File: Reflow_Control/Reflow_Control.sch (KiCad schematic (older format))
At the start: 36 parts

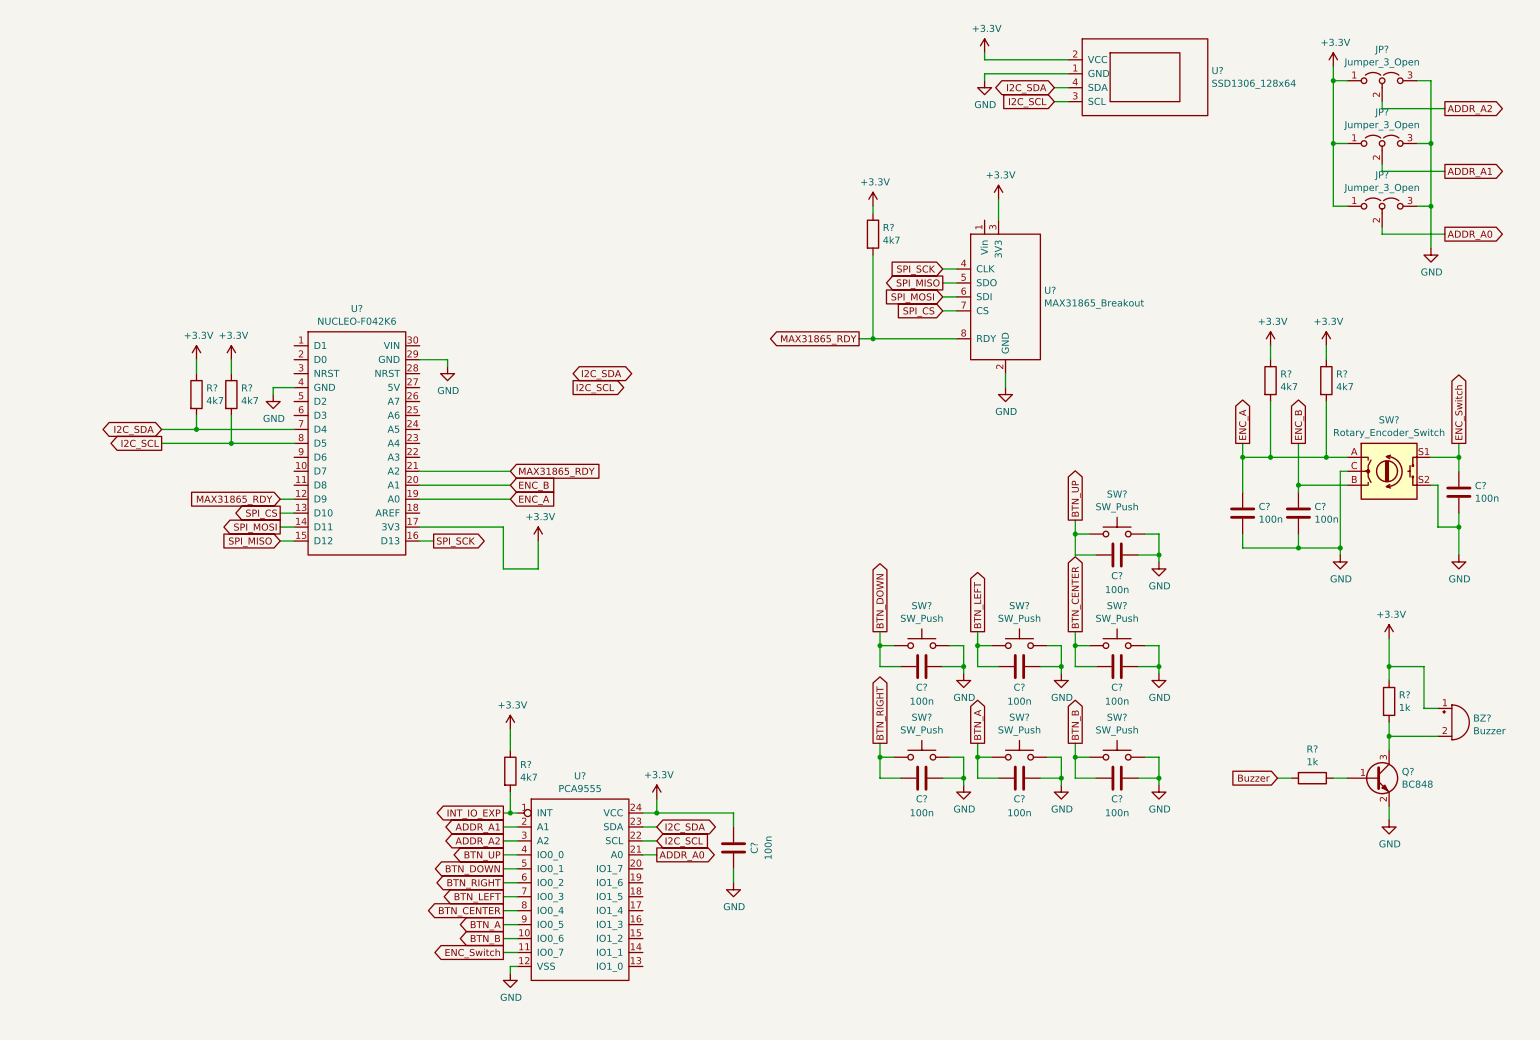
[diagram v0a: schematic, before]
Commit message: work on naming
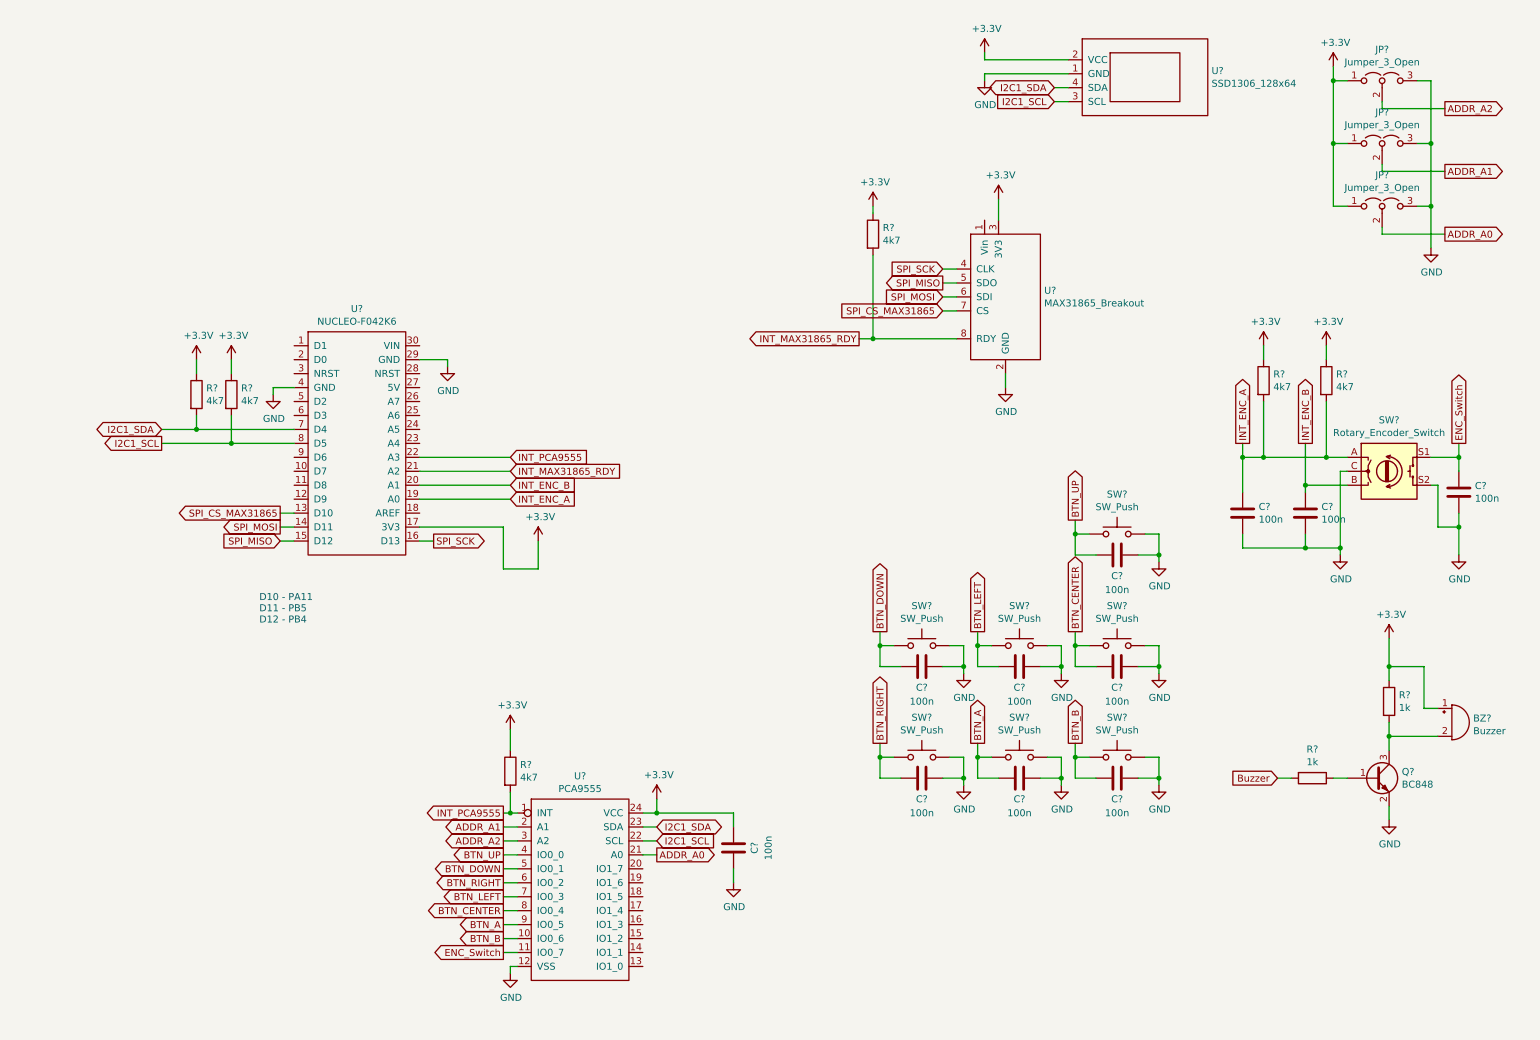
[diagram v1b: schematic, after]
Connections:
- net INT_IO_EXP is gone; now on net INT_PCA9555: R?.2, U?.1 (INT)
- net INT_PCA9555: now reaches U?.22 (A3)
- net ENC_A renamed INT_ENC_A
- net ENC_B renamed INT_ENC_B
- net I2C_SCL renamed I2C1_SCL
- net I2C_SDA renamed I2C1_SDA
- net MAX31865_RDY renamed INT_MAX31865_RDY
- net INT_MAX31865_RDY: no longer U?.12 (D9)
- net SPI_CS renamed SPI_CS_MAX31865
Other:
- note added: "D10 - PA11\nD11 - PB5\nD12 - PB4\n"
- moved on the sheet: C?, R?
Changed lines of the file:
@@
 L Device:R R?
 U 1 1 5F9458E6
-P 9450 3150
-F 0 "R?" H 9520 3196 50  0000 L CNN
-F 1 "4k7" H 9520 3105 50  0000 L CNN
-F 2 "Resistor_SMD:R_1206_3216Metric_Pad1.42x1.75mm_HandSolder" V 9380 3150 50  0001 C CNN
-F 3 "~" H 9450 3150 50  0001 C CNN
-F 4 "Rhom" H 9450 3150 50  0001 C CNN "Man"
-F 5 "KTR18EZPF4701" H 9450 3150 50  0001 C CNN "Man no"
-F 6 "Digikey" H 9450 3150 50  0001 C CNN "Dist"
-F 7 "RHM4.7KAICT-ND" H 9450 3150 50  0001 C CNN "Dist no"
-	1    9450 3150
+P 9400 3150
+F 0 "R?" H 9470 3196 50  0000 L CNN
+F 1 "4k7" H 9470 3105 50  0000 L CNN
+F 2 "Resistor_SMD:R_1206_3216Metric_Pad1.42x1.75mm_HandSolder" V 9330 3150 50  0001 C CNN
+F 3 "~" H 9400 3150 50  0001 C CNN
+F 4 "Rhom" H 9400 3150 50  0001 C CNN "Man"
+F 5 "KTR18EZPF4701" H 9400 3150 50  0001 C CNN "Man no"
+F 6 "Digikey" H 9400 3150 50  0001 C CNN "Dist"
+F 7 "RHM4.7KAICT-ND" H 9400 3150 50  0001 C CNN "Dist no"
+	1    9400 3150
 	1    0    0    -1
 $EndComp
@@
 L Device:C C?
 U 1 1 5F947CDD
-P 9650 4100
-F 0 "C?" H 9765 4146 50  0000 L CNN
-F 1 "100n" H 9765 4055 50  0000 L CNN
-F 2 "Capacitor_SMD:C_0805_2012Metric_Pad1.15x1.40mm_HandSolder" H 9688 3950 50  0001 C CNN
-F 3 "~" H 9650 4100 50  0001 C CNN
-F 4 "Samsung" H 9650 4100 50  0001 C CNN "Man"
-F 5 "CL21B104KACNNNC" H 9650 4100 50  0001 C CNN "Man nno"
-F 6 "Digikey" H 9650 4100 50  0001 C CNN "Dist"
-F 7 "1276-1099-1-ND" H 9650 4100 50  0001 C CNN "Dist no"
-	1    9650 4100
+P 9700 4100
+F 0 "C?" H 9815 4146 50  0000 L CNN
+F 1 "100n" H 9815 4055 50  0000 L CNN
+F 2 "Capacitor_SMD:C_0805_2012Metric_Pad1.15x1.40mm_HandSolder" H 9738 3950 50  0001 C CNN
+F 3 "~" H 9700 4100 50  0001 C CNN
+F 4 "Samsung" H 9700 4100 50  0001 C CNN "Man"
+F 5 "CL21B104KACNNNC" H 9700 4100 50  0001 C CNN "Man nno"
+F 6 "Digikey" H 9700 4100 50  0001 C CNN "Dist"
+F 7 "1276-1099-1-ND" H 9700 4100 50  0001 C CNN "Dist no"
+	1    9700 4100
 	1    0    0    -1
 $EndComp
@@
 	9950 3800 10000 3800
 Wire Wire Line
-	10000 3900 9650 3900
-Wire Wire Line
-	9650 3900 9650 3950
+	10000 3900 9700 3900
+Wire Wire Line
+	9700 3900 9700 3950
 Wire Wire Line
 	10000 3700 9850 3700
@@
 	9250 4250 9250 4350
 Wire Wire Line
-	9250 4350 9650 4350
+	9250 4350 9700 4350
 Connection ~ 9950 4350
 Wire Wire Line
 	9950 4350 9950 3800
 Wire Wire Line
-	9650 4250 9650 4350
-Connection ~ 9650 4350
-Wire Wire Line
-	9650 4350 9950 4350
+	9700 4250 9700 4350
+Connection ~ 9700 4350
+Wire Wire Line
+	9700 4350 9950 4350
 Text GLabel 9250 3600 1    50   Output ~ 0
-ENC_A
-Text GLabel 9650 3600 1    50   Output ~ 0
-ENC_B
+INT_ENC_A
+Text GLabel 9700 3600 1    50   Output ~ 0
+INT_ENC_B
 Wire Wire Line
 	9250 3600 9250 3700
 Connection ~ 9250 3700
 Wire Wire Line
-	9650 3600 9650 3900
-Connection ~ 9650 3900
+	9700 3600 9700 3900
+Connection ~ 9700 3900
 Text GLabel 10800 3600 1    50   Output ~ 0
 ENC_Switch
@@
 $EndComp
 Wire Wire Line
-	9450 3300 9450 3700
-Connection ~ 9450 3700
-Wire Wire Line
-	9450 3700 9250 3700
+	9400 3300 9400 3700
+Connection ~ 9400 3700
+Wire Wire Line
+	9400 3700 9250 3700
 Wire Wire Line
 	9850 3300 9850 3700
 Connection ~ 9850 3700
 Wire Wire Line
-	9850 3700 9450 3700
+	9850 3700 9400 3700
 $Comp
 L power:+3.3V #PWR?
 U 1 1 5F9E4634
-P 9450 2900
-F 0 "#PWR?" H 9450 2750 50  0001 C CNN
-F 1 "+3.3V" H 9465 3073 50  0000 C CNN
-F 2 "" H 9450 2900 50  0001 C CNN
-F 3 "" H 9450 2900 50  0001 C CNN
-	1    9450 2900
+P 9400 2900
+F 0 "#PWR?" H 9400 2750 50  0001 C CNN
+F 1 "+3.3V" H 9415 3073 50  0000 C CNN
+F 2 "" H 9400 2900 50  0001 C CNN
+F 3 "" H 9400 2900 50  0001 C CNN
+	1    9400 2900
 	1    0    0    -1
 $EndComp
@@
 	9850 2900 9850 3000
 Wire Wire Line
-	9450 3000 9450 2900
+	9400 3000 9400 2900
 $Comp
 L Jumper:Jumper_3_Open JP?
@@
 Connection ~ 5050 6250
 Text GLabel 3950 6250 0    50   Output ~ 0
-INT_IO_EXP
+INT_PCA9555
 Wire Wire Line
 	4050 6250 4000 6250
@@
 	4000 5650 4000 5800
 Text GLabel 5050 6450 2    50   Input ~ 0
-I2C_SCL
+I2C1_SCL
 Text GLabel 5050 6350 2    50   BiDi ~ 0
-I2C_SDA
+I2C1_SDA
 Wire Wire Line
 	5050 6450 4950 6450
@@
 	5050 6350 4950 6350
 Text GLabel 1500 3500 0    50   BiDi ~ 0
-I2C_SDA
+I2C1_SDA
 Text GLabel 1500 3600 0    50   Output ~ 0
-I2C_SCL
+I2C1_SCL
 $Comp
 L Device:R R?
@@
 	3550 3000 3550 3050
 Text GLabel 7900 1050 0    50   BiDi ~ 0
-I2C_SDA
+I2C1_SDA
 Text GLabel 7900 1150 0    50   Input ~ 0
-I2C_SCL
+I2C1_SCL
 Wire Wire Line
 	7900 1050 8000 1050
@@
 SPI_SCK
 Text GLabel 2350 4100 0    50   Output ~ 0
-SPI_CS
+SPI_CS_MAX31865
 Wire Wire Line
 	2350 4100 2450 4100
 Text GLabel 7100 2650 0    50   Input ~ 0
-SPI_CS
+SPI_CS_MAX31865
 Wire Wire Line
 	7100 2650 7200 2650
@@
 Wire Wire Line
 	7200 2450 7100 2450
-Text GLabel 2350 4000 0    50   Input ~ 0
-MAX31865_RDY
 Wire Wire Line
 	7100 2550 7200 2550
-Wire Wire Line
-	2350 4000 2450 4000
 Text GLabel 6500 2850 0    50   Output ~ 0
-MAX31865_RDY
+INT_MAX31865_RDY
 Wire Wire Line
 	6500 2850 6600 2850
@@
 	6600 1900 6600 1950
 Text GLabel 4000 4000 2    50   Input ~ 0
-ENC_A
+INT_ENC_A
 Text GLabel 4000 3900 2    50   Input ~ 0
-ENC_B
+INT_ENC_B
 Wire Wire Line
 	3350 3900 4000 3900
@@
 	4200 4500 4200 4300
 Text GLabel 4000 3800 2    50   Input ~ 0
-MAX31865_RDY
+INT_MAX31865_RDY
 Wire Wire Line
 	4000 3800 3350 3800
@@
 Wire Wire Line
 	7500 1850 7500 2000
-Text GLabel 4450 3100 2    50   BiDi ~ 0
-I2C_SDA
-Text GLabel 4450 3200 2    50   Output ~ 0
-I2C_SCL
+Text Notes 2200 4900 0    50   ~ 0
+D10 - PA11\nD11 - PB5\nD12 - PB4\n
+Text GLabel 4000 3700 2    50   Input ~ 0
+INT_PCA9555
+Wire Wire Line
+	4000 3700 3350 3700
 $EndSCHEMATC

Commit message: naming signals
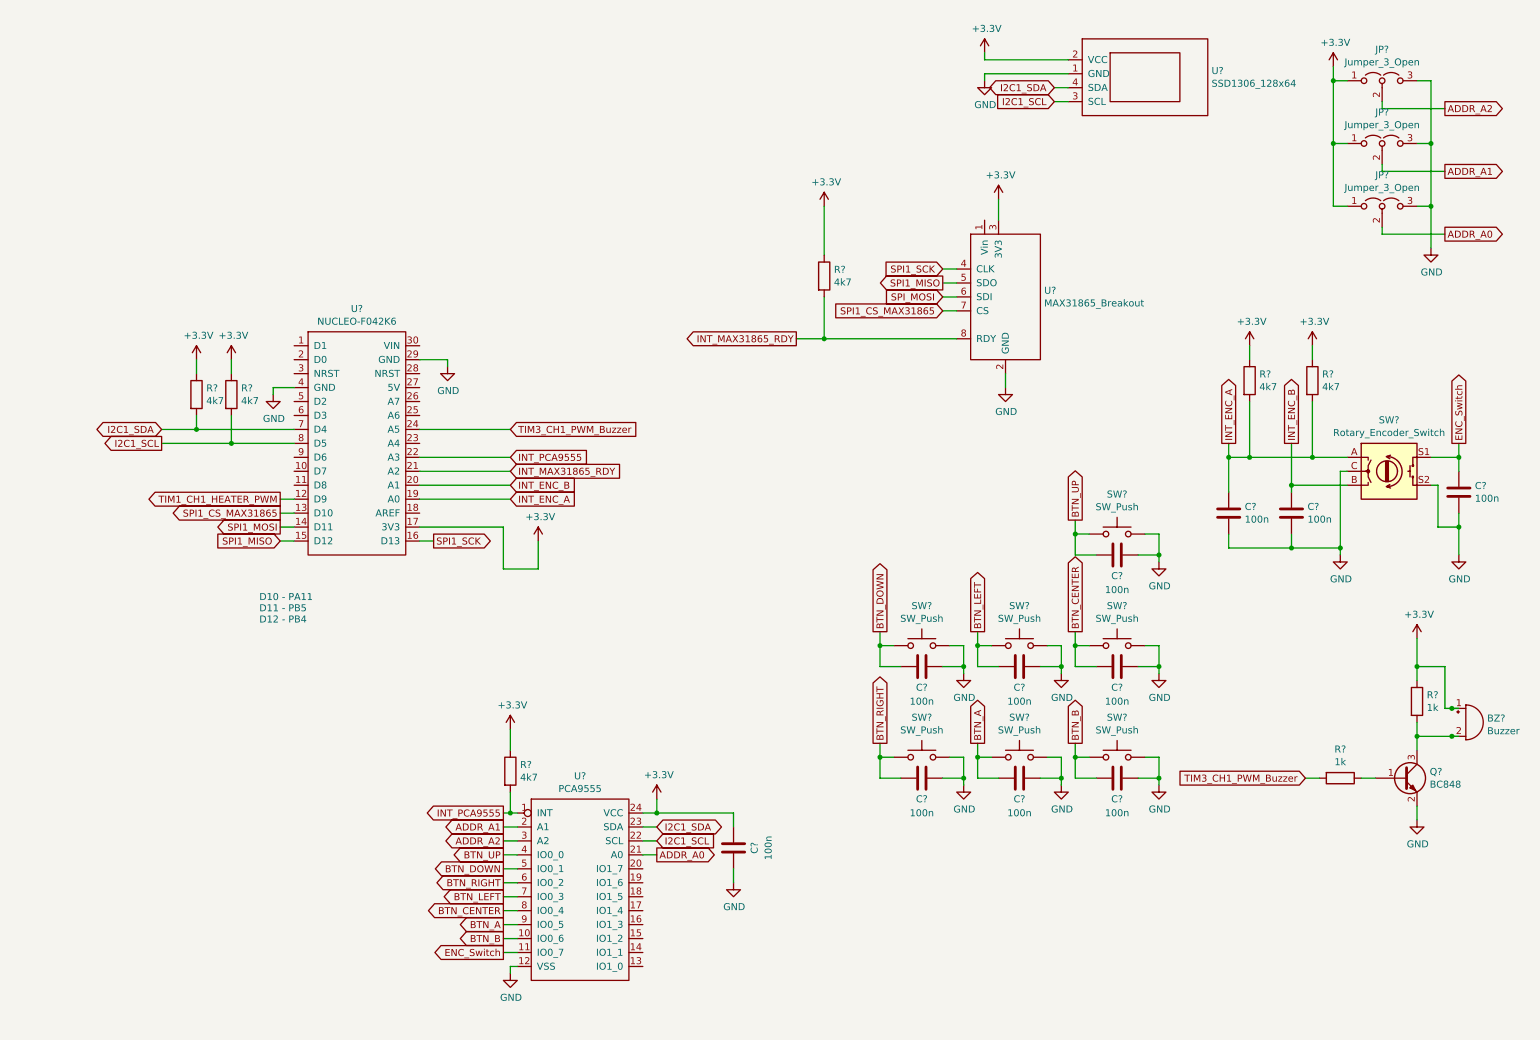
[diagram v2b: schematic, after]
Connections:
- net Buzzer is gone; now on net TIM3_CH1_PWM_Buzzer: R?.2
- net SPI_MOSI: no longer U?.14 (D11)
- net TIM1_CH1_HEATER_PWM: now reaches U?.12 (D9)
- net TIM3_CH1_PWM_Buzzer: now reaches U?.24 (A5)
- net SPI_CS_MAX31865 renamed SPI1_CS_MAX31865
- net SPI_MISO renamed SPI1_MISO
- net SPI_SCK renamed SPI1_SCK
- new net SPI1_MOSI: U?.14 (D11)
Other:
- moved on the sheet: BZ?, C?, Q?, R?

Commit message: Updated version with Edwin & Kerem 29.11.2020 Only Schema
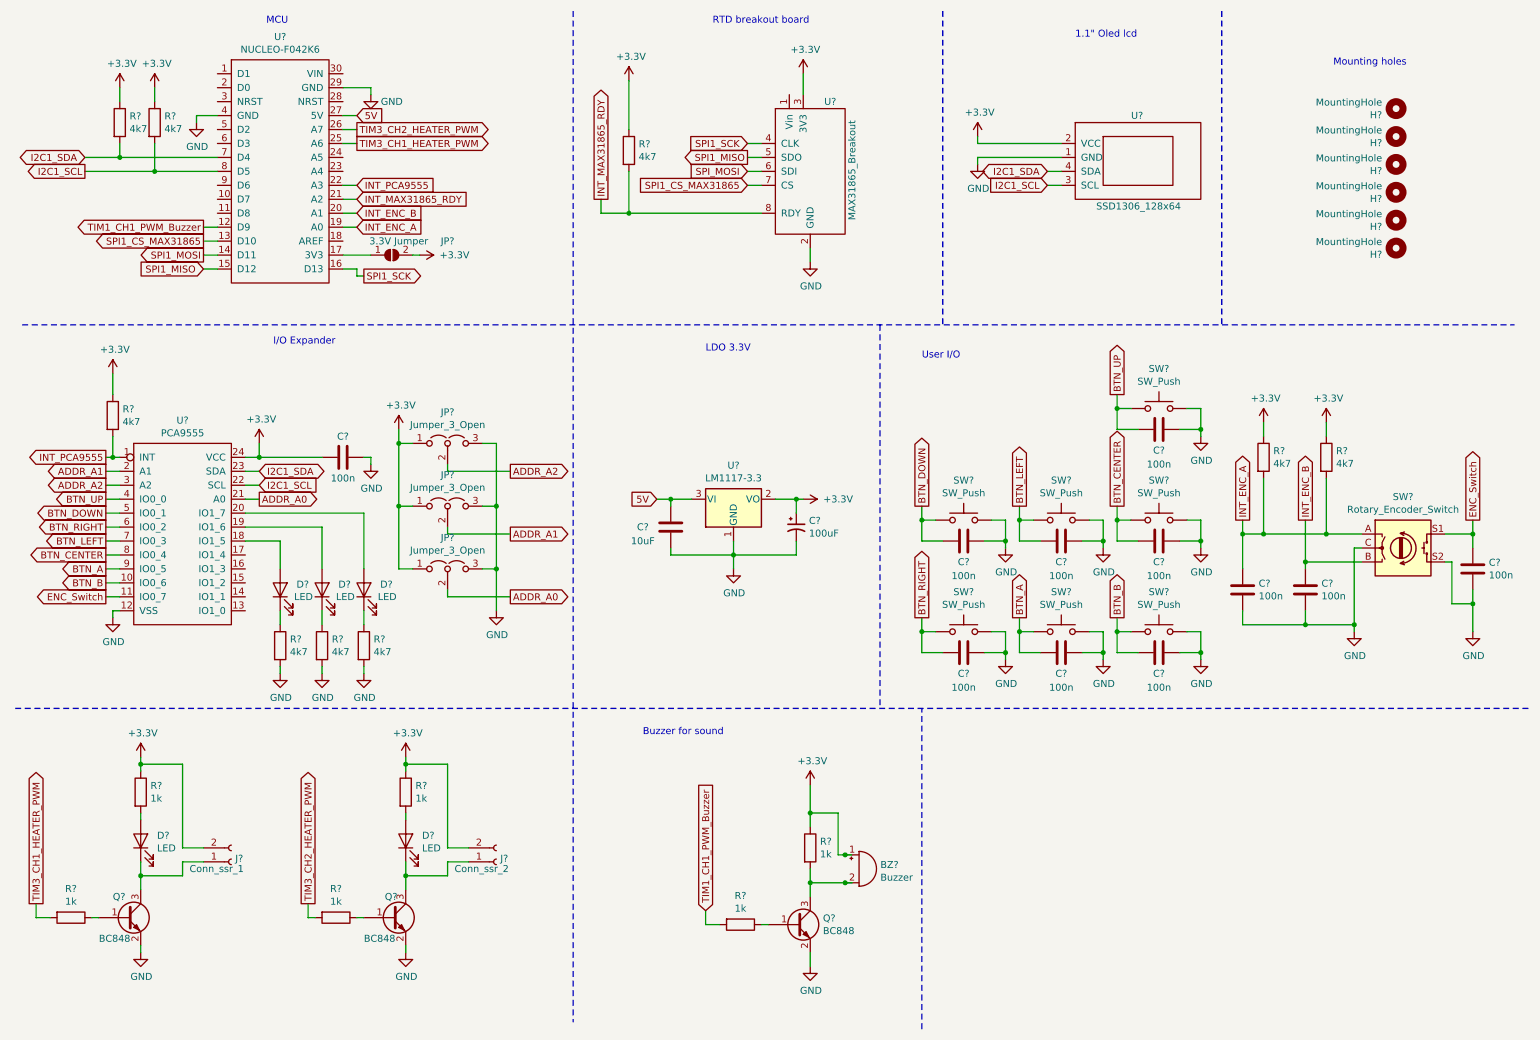
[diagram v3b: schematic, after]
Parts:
- added C?: 10uF, Capacitor_SMD:C_0805_2012Metric_Pad1.15x1.40mm_HandSolder, symbol Device:C
- added C?: 100uF, PCE3853CT-ND, symbol Device:CP1_Small
- added D? (x5): LED, LED_SMD:LED_1206_3216Metric_Pad1.42x1.75mm_HandSolder, symbol Device:LED
- added H? (x6): MountingHole, MountingHole:MountingHole_2.5mm_Pad, symbol Mechanical:MountingHole
- added J?: Conn_ssr_2, Connector_Phoenix_MC_HighVoltage:PhoenixContact_MC_1,5_2-G-5.08_1x02_P5.08mm_Horizontal, symbol Connector:Conn_01x02_Female
- added J?: Conn_ssr_1, Connector_Phoenix_MC_HighVoltage:PhoenixContact_MC_1,5_2-G-5.08_1x02_P5.08mm_Horizontal, symbol Connector:Conn_01x02_Female
- added JP?: 3.3V Jumper, Jumper:SolderJumper-2_P1.3mm_Open_RoundedPad1.0x1.5mm, symbol Jumper:SolderJumper_2_Open
- added Q? (x2): BC848, Package_TO_SOT_SMD:SOT-23, symbol Transistor_BJT:BC848
- added R? (x4): 1k, Resistor_SMD:R_1206_3216Metric_Pad1.42x1.75mm_HandSolder, symbol Device:R
- added R? (x3): 4k7, Resistor_SMD:R_1206_3216Metric_Pad1.42x1.75mm_HandSolder, symbol Device:R
- added U?: LM1117-3.3, symbol Regulator_Linear:LM1117-3.3
- SW?: footprint (none) -> Rotary_Encoder:RotaryEncoder_Alps_EC11E_Vertical_H20mm; Dist no PEC11L-4220F-S0015-ND -> PEC12R-4220F-S0024-ND; Man no PEC11L-4220F-S0015 -> PEC12R-4220F-S0024
- U?: footprint MY_FOOTPRINT:MAX31865_Breakout -> Connector_PinHeader_2.54mm:PinHeader_1x08_P2.54mm_Vertical
- U?: footprint (none) -> Connector_PinHeader_2.54mm:PinHeader_1x04_P2.54mm_Vertical
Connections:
- net +3V3: now also C?.2, C?.1, J?.2 (Pin_2), J?.2 (Pin_2), JP?.2 (B), R?.1, R?.1, U?.2 (VO); no longer C?.1, U?.17 (3V3)
- net GND: now also C?.1, C?.2, C?.2, Q?.2 (E), Q?.2 (E), R?.2, R?.2, R?.2, U?.1 (GND); no longer C?.2
- net TIM3_CH1_HEATER_PWM: now reaches U?.25 (A6)
- net TIM3_CH1_HEATER_PWM: now also R?.2
- net TIM3_CH2_HEATER_PWM: now reaches U?.26 (A7)
- net TIM3_CH2_HEATER_PWM: now also R?.2
- net 5V: now reaches U?.27 (5V)
- net 5V: now also C?.1, U?.3 (VI)
- net at U?.18 (IO1_5): now also D?.2 (A)
- net at U?.19 (IO1_6): now also D?.2 (A)
- net at U?.20 (IO1_7): now also D?.2 (A)
- net TIM1_CH1_HEATER_PWM renamed TIM1_CH1_PWM_Buzzer
- net TIM1_CH1_PWM_Buzzer: now also R?.2
- net TIM3_CH1_PWM_Buzzer: no longer names the net of U?.24 (A5)
- net TIM3_CH1_PWM_Buzzer: no longer R?.2
- new net: JP?.1 (A), U?.17 (3V3)
- new net: Q?.1 (B), R?.1 (x2)
- new net: D?.1 (K), J?.1 (Pin_1), Q?.3 (C) (x2)
- new net: D?.2 (A), R?.2 (x2)
- new net: D?.1 (K), R?.1 (x3)
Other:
- note added: "1.1" Oled lcd"
- note added: "Buzzer for sound"
- note added: "I/O Expander"
- note added: "LDO 3.3V"
- note added: "MCU"
- note added: "Mounting holes"
- note added: "RTD breakout board"
- note added: "User I/O"
- note removed: "D10 - PA11\nD11 - PB5\nD12 - PB4\n"
- moved on the sheet: BZ?, C?, JP?, Q?, R?, SW?, U?
